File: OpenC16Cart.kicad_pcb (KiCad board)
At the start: 2 copper layers, 52 x 65 mm, 16 parts, among them J1 CONN_02X03, J11 CONN_01X03, J12 CONN_01X03, J2 CONN_01X03, J21 CONN_01X03, J22 CONN_01X03, J3 CONN_01X03, J4 CONN_02X03, J5 CONN_01X03, J6 CONN_01X03, J7 C16-Exp-Port, U1 27512 - LO ROM, U2 27512 - HI ROM

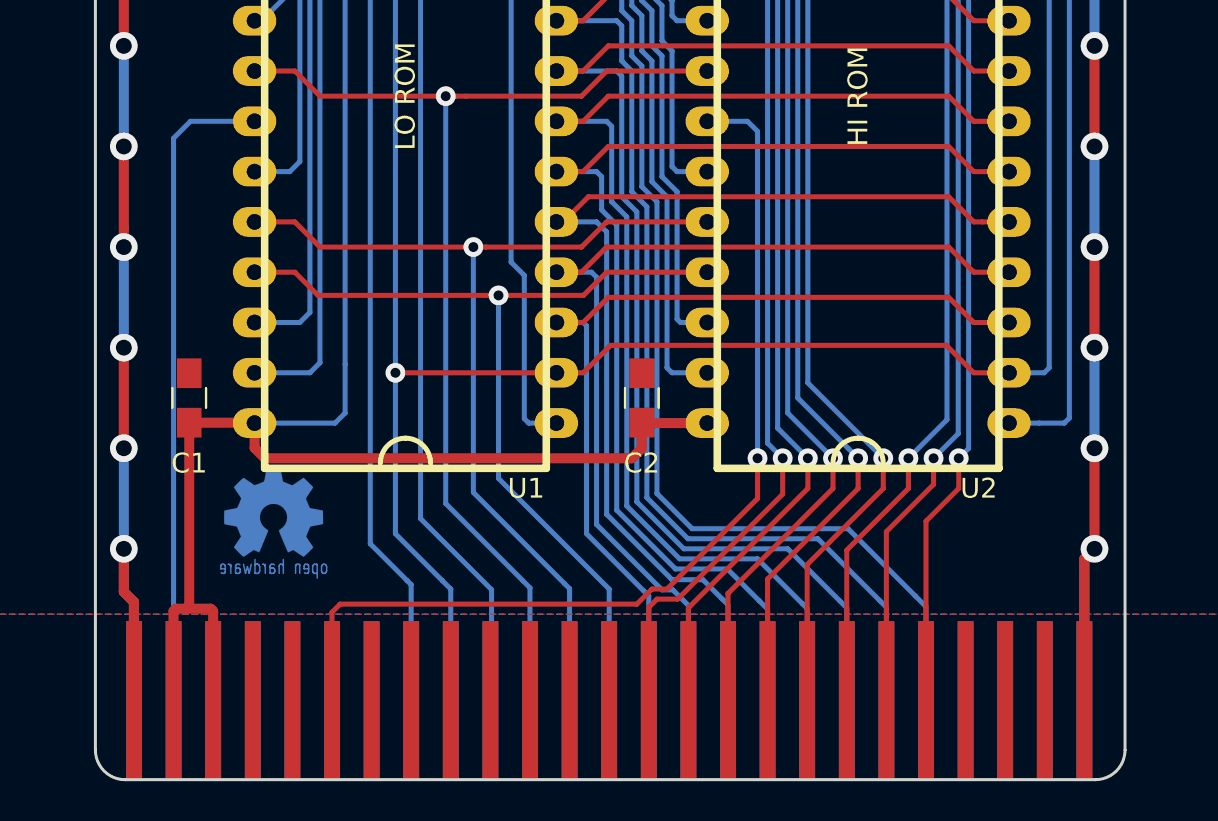
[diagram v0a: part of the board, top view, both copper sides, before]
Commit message: Final touches for V3
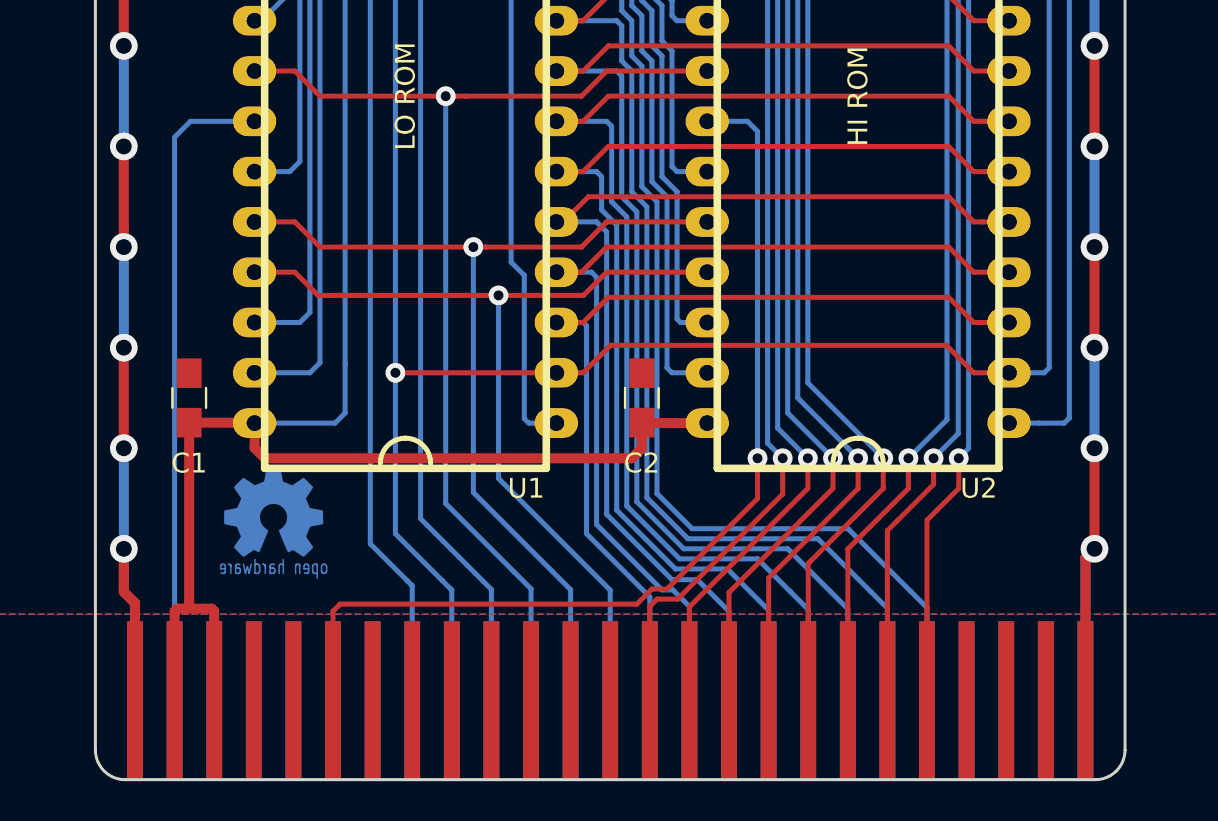
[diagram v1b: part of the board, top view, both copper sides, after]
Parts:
- moved J7 0.05 mm to (147.5, 124.5)
